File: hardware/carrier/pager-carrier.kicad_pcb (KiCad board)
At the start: 2 copper layers, 97 parts, among them J10 HAPTIC, J11 EXT_LED, J12 PIEZ, J13 USB4235, J14 BATTERY, J5 PANEL, J9 CARDKB, M2 Walter, Q2 AO3401A, Q6 UMH3N, Q7 AO3400A, Q8 MMBT3904, SW3 SKQGAFE010, SW4 JS102011SAQN, U12 CP2102N-A02-GQFN24, U13 SN74LVC2G126DCUR, U14 DRV2605LDGSR, U15 LIS2DW12TR, U16 MAX17048G+T10, U2 BQ25185DLHR, U4 TPS62840DLCR

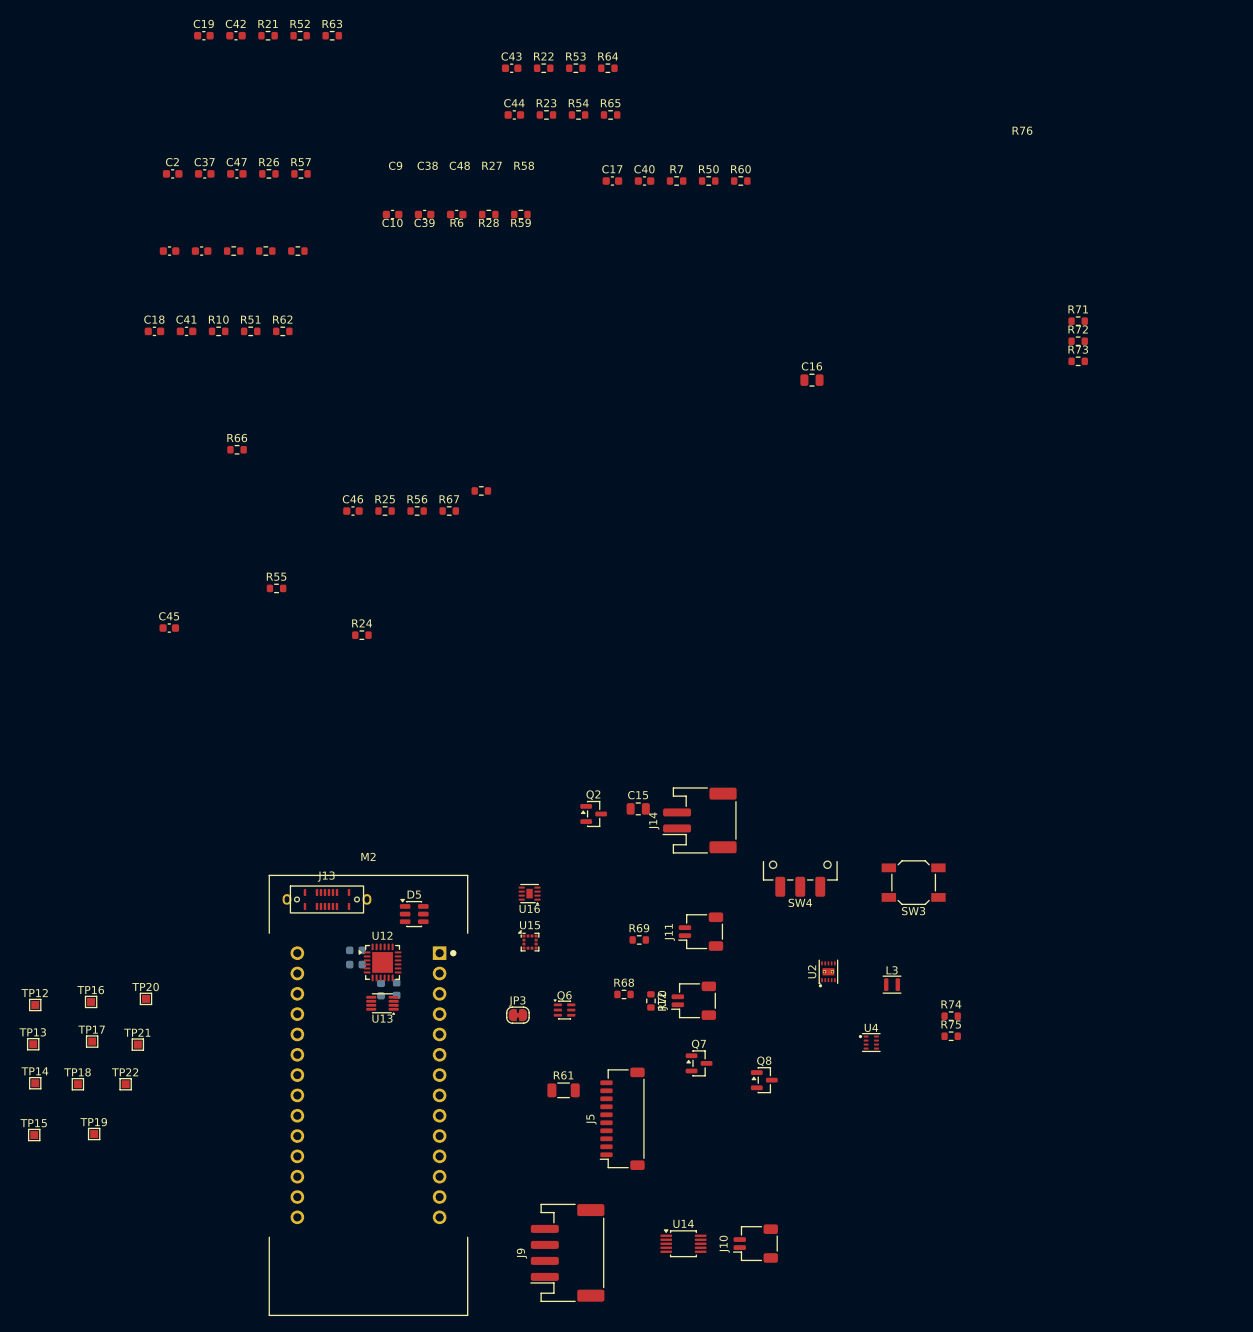
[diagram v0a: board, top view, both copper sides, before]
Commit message: Attempt to layout the PCB
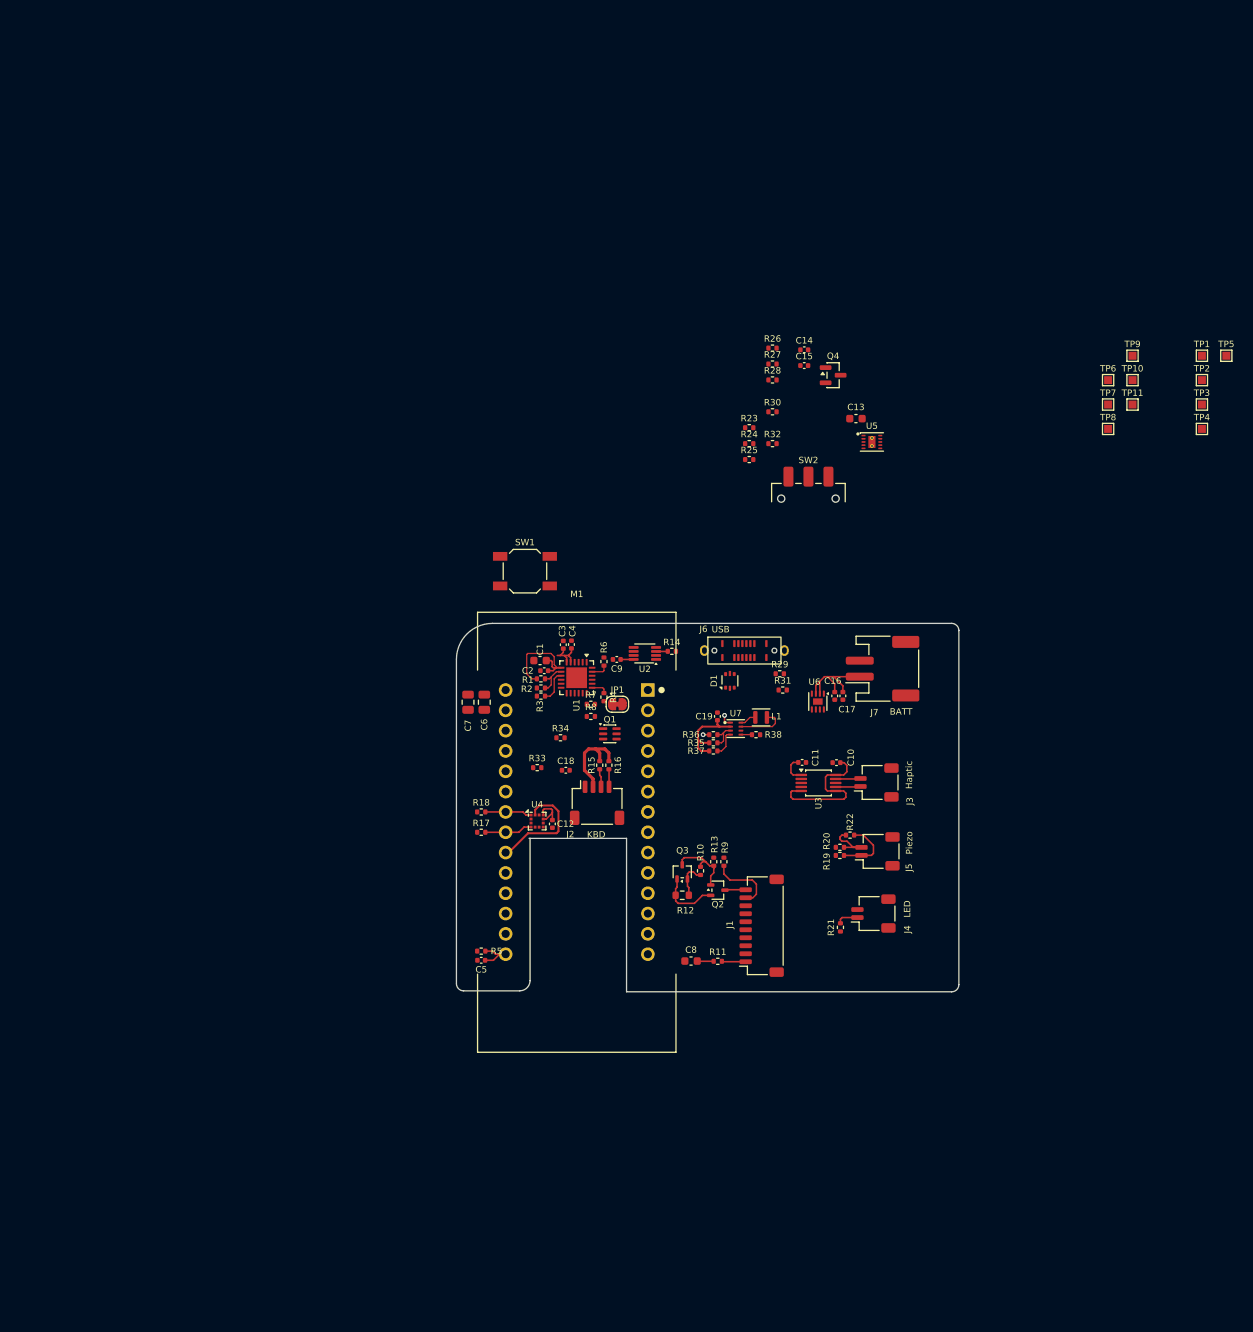
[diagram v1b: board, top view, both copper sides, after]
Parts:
- removed C33, C36: 4.7uF, Capacitor_SMD:C_0603_1608Metric
- removed C34, C35, C37, C39, C42, C45, C46: 100nF, Capacitor_SMD:C_0603_1608Metric
- removed C38, C40, C43, C47, C48: 10uF, Capacitor_SMD:C_0603_1608Metric
- removed C41, C44: 1uF, Capacitor_SMD:C_0603_1608Metric
- removed D5: USBLC6-2SC6, Package_TO_SOT_SMD:SOT-23-6
- removed J10: HAPTIC, Connector_JST:JST_SH_SM02B-SRSS-TB_1x02-1MP_P1.00mm_Horizontal
- removed J11: EXT_LED, Connector_JST:JST_SH_SM02B-SRSS-TB_1x02-1MP_P1.00mm_Horizontal
- removed J12: PIEZ, Connector_JST:JST_SH_SM02B-SRSS-TB_1x02-1MP_P1.00mm_Horizontal
- removed J13: USB4235, pager-carrier:USB_C_Receptacle_GCT_USB4235_Vertical
- removed J14: BATTERY, Connector_JST:JST_PH_S2B-PH-SM4-TB_1x02-1MP_P2.00mm_Horizontal
- removed J9: CARDKB, Connector_JST:JST_PH_S4B-PH-SM4-TB_1x04-1MP_P2.00mm_Horizontal
- removed JP3: auto-boot, Jumper:SolderJumper-2_P1.3mm_Bridged_RoundedPad1.0x1.5mm
- removed L3: 2.2uH, Inductor_SMD:L_Murata_DFE201610P
- removed M2: Walter, pager-carrier:Walter_Module_2x14_THT
- removed Q6: UMH3N, Package_TO_SOT_SMD:SOT-363_SC-70-6
- removed Q7: AO3400A, Package_TO_SOT_SMD:SOT-23
- removed Q8: MMBT3904, Package_TO_SOT_SMD:SOT-23
- removed R50: 22.1k, Resistor_SMD:R_0603_1608Metric
- removed R51: 47.5k, Resistor_SMD:R_0603_1608Metric
- removed R52, R58: 1k, Resistor_SMD:R_0603_1608Metric
- removed R53, R54, R55, R59, R72, R75: 100k, Resistor_SMD:R_0603_1608Metric
- removed R56, R57, R62: 10k, Resistor_SMD:R_0603_1608Metric
- removed R60: 15R, Resistor_SMD:R_0603_1608Metric
- removed R61: 0R, Resistor_SMD:R_1206_3216Metric
- removed R63, R64, R65, R66: 4.7k, Resistor_SMD:R_0603_1608Metric
- removed R67, R68: 220R, Resistor_SMD:R_0603_1608Metric
- removed R69: 330R, Resistor_SMD:R_0603_1608Metric
- removed R70: 1M, Resistor_SMD:R_0603_1608Metric
- removed R71: 56k, Resistor_SMD:R_0603_1608Metric
- removed R73, R74: 0R, Resistor_SMD:R_0603_1608Metric
- removed R76: 267k, Resistor_SMD:R_0603_1608Metric
- removed SW3: SKQGAFE010, Button_Switch_SMD:SW_SPST_SKQG_WithoutStem
- removed SW4: JS102011SAQN, Button_Switch_SMD:SW_SPDT_CK_JS102011SAQN
- removed TP12: AWK_EN_N, TestPoint:TestPoint_Pad_1.0x1.0mm
- removed TP13: TP_IO1, TestPoint:TestPoint_Pad_1.0x1.0mm
- removed TP14: TP_IO5, TestPoint:TestPoint_Pad_1.0x1.0mm
- removed TP15: FL_BTN, TestPoint:TestPoint_Pad_1.0x1.0mm
- removed TP16: 3V3_AWK, TestPoint:TestPoint_Pad_1.0x1.0mm
- removed TP17: GND, TestPoint:TestPoint_Pad_1.0x1.0mm
- removed TP18: VBUS, TestPoint:TestPoint_Pad_1.0x1.0mm
- removed TP19: SYS, TestPoint:TestPoint_Pad_1.0x1.0mm
- removed TP20: SYS_SW, TestPoint:TestPoint_Pad_1.0x1.0mm
- removed TP21: VBAT, TestPoint:TestPoint_Pad_1.0x1.0mm
- removed TP22: 3V3, TestPoint:TestPoint_Pad_1.0x1.0mm
- removed U12: CP2102N-A02-GQFN24, Package_DFN_QFN:QFN-24-1EP_4x4mm_P0.5mm_EP2.6x2.6mm
- removed U13: SN74LVC2G126DCUR, Package_SO:VSSOP-8_2.3x2mm_P0.5mm
- removed U14: DRV2605LDGSR, Package_SO:TSSOP-10_3x3mm_P0.5mm
- removed U15: LIS2DW12TR, Package_LGA:LGA-12_2x2mm_P0.5mm
- removed U16: MAX17048G+T10, Package_DFN_QFN:TDFN-8-1EP_2x2mm_P0.5mm_EP0.8x1.2mm
- added C1: 4.7uF, Capacitor_SMD:C_0603_1608Metric, F.Cu at (82.2, 63.2)
- added C11: 1uF, Capacitor_SMD:C_0402_1005Metric, F.Cu at (114.9, 76.0)
- added C12: 100nF, Capacitor_SMD:C_0402_1005Metric, F.Cu at (83.7, 83.7)
- added C13: 1uF/25V, Capacitor_SMD:C_0603_1608Metric, F.Cu at (121.6, 33.0)
- added C14: 22nF, Capacitor_SMD:C_0402_1005Metric, F.Cu at (115.2, 24.4)
- added C3: 100nF, Capacitor_SMD:C_0402_1005Metric, F.Cu at (85.1, 61.3)
- added C4: 4.7uF, Capacitor_SMD:C_0402_1005Metric, F.Cu at (86.1, 61.2)
- added C5: 100nF, Capacitor_SMD:C_0402_1005Metric, F.Cu at (74.8, 100.7)
- added C6: 100uF, Capacitor_SMD:C_0805_2012Metric, F.Cu at (75.2, 68.5)
- added C7: 100uF, Capacitor_SMD:C_0805_2012Metric, F.Cu at (73.2, 68.5)
- added C8: 10uF, Capacitor_SMD:C_0603_1608Metric, F.Cu at (101.0, 100.8)
- added D1: USBLC6-2P6, Package_TO_SOT_SMD:SOT-666, F.Cu at (105.9, 65.8)
- added J1: PANEL, Connector_JST:JST_SH_SM10B-SRSS-TB_1x10-1MP_P1.00mm_Horizontal, F.Cu at (109.9, 96.4)
- added J2: CARDKB, Connector_JST:JST_SH_SM04B-SRSS-TB_1x04-1MP_P1.00mm_Horizontal, F.Cu at (89.3, 81.0)
- added J3: HAPTIC, Connector_JST:JST_SH_SM02B-SRSS-TB_1x02-1MP_P1.00mm_Horizontal, F.Cu at (124.2, 78.5)
- added J4: EXT_LED, Connector_JST:JST_SH_SM02B-SRSS-TB_1x02-1MP_P1.00mm_Horizontal, F.Cu at (123.8, 94.9)
- added J6: USB4235, pager-carrier:USB_C_Receptacle_GCT_USB4235_Vertical, F.Cu at (107.7, 62.0)
- added J7: BATTERY, Connector_JST:JST_PH_S2B-PH-SM4-TB_1x02-1MP_P2.00mm_Horizontal, F.Cu at (125.0, 64.3)
- added JP1: auto-boot, Jumper:SolderJumper-2_P1.3mm_Bridged_RoundedPad1.0x1.5mm, F.Cu at (91.8, 68.7)
- added L1: 2.2uH, Inductor_SMD:L_Murata_DFE201610P, F.Cu at (109.8, 70.4)
- added M1: Walter, pager-carrier:Walter_Module_2x14_THT, F.Cu at (86.7, 83.4)
- added Q1: UMH3N, Package_TO_SOT_SMD:SOT-363_SC-70-6, F.Cu at (90.9, 72.4)
- added Q3: MMST3904, Package_TO_SOT_SMD:SOT-323_SC-70, F.Cu at (99.9, 89.7)
- added Q4: AO3401A, Package_TO_SOT_SMD:SOT-23, F.Cu at (118.8, 27.6)
- added R1: 22.1k, Resistor_SMD:R_0402_1005Metric, F.Cu at (82.3, 65.5)
- added R11: 0R, Resistor_SMD:R_0402_1005Metric, F.Cu at (104.4, 100.8)
- added R12: 15R, Resistor_SMD:R_0603_1608Metric, F.Cu at (99.9, 92.6)
- added R13: 0R, Resistor_SMD:R_0402_1005Metric, F.Cu at (105.1, 88.4)
- added R14: 10k, Resistor_SMD:R_0402_1005Metric, F.Cu at (98.6, 62.1)
- added R15: 4.7k, Resistor_SMD:R_0402_1005Metric, F.Cu at (89.6, 76.3)
- added R16: 4.7k, Resistor_SMD:R_0402_1005Metric, F.Cu at (90.8, 76.3)
- added R17: 4.7k, Resistor_SMD:R_0402_1005Metric, F.Cu at (74.8, 84.7)
- added R18: 4.7k, Resistor_SMD:R_0402_1005Metric, F.Cu at (74.8, 82.2)
- added R19: 220R, Resistor_SMD:R_0402_1005Metric, F.Cu at (119.6, 87.6)
- added R2: 47.5k, Resistor_SMD:R_0402_1005Metric, F.Cu at (82.3, 66.7)
- added R20: 220R, Resistor_SMD:R_0402_1005Metric, F.Cu at (119.6, 86.6)
- added R29: 5.1k, Resistor_SMD:R_0402_1005Metric, F.Cu at (112.1, 64.9)
- added R3: 1k, Resistor_SMD:R_0402_1005Metric, F.Cu at (82.3, 67.7)
- added R30: 10k, Resistor_SMD:R_0402_1005Metric, F.Cu at (111.2, 32.2)
- added R31: 5.1k, Resistor_SMD:R_0402_1005Metric, F.Cu at (112.5, 66.9)
- added R32: 2.2M, Resistor_SMD:R_0402_1005Metric, F.Cu at (111.2, 36.1)
- added R33: 56k, Resistor_SMD:R_0402_1005Metric, F.Cu at (81.8, 76.6)
- added R34: 100k, Resistor_SMD:R_0402_1005Metric, F.Cu at (84.7, 72.9)
- added R35: 0R, Resistor_SMD:R_0402_1005Metric, F.Cu at (103.8, 73.5)
- added R36: 0R, Resistor_SMD:R_0402_1005Metric, F.Cu at (103.8, 72.5)
- added R37: 100k, Resistor_SMD:R_0402_1005Metric, F.Cu at (103.8, 74.5)
- added R38: 267k, Resistor_SMD:R_0402_1005Metric, F.Cu at (109.2, 72.5)
- added R4: 100k, Resistor_SMD:R_0402_1005Metric, F.Cu at (90.1, 67.8)
- added R5: 100k, Resistor_SMD:R_0402_1005Metric, F.Cu at (74.8, 99.6)
- added R8: 10k, Resistor_SMD:R_0402_1005Metric, F.Cu at (88.5, 70.2)
- added R9: 1k, Resistor_SMD:R_0402_1005Metric, F.Cu at (103.9, 88.4)
- added SW1: SKQGAFE010, Button_Switch_SMD:SW_SPST_SKQG_WithoutStem, F.Cu at (80.3, 52.1)
- added SW2: JS102011SAQN, Button_Switch_SMD:SW_SPDT_CK_JS102011SAQN, F.Cu at (115.7, 43.0)
- added TP1: AWK_EN_N, TestPoint:TestPoint_Pad_1.0x1.0mm, F.Cu at (164.9, 25.1)
- added TP10: VBAT, TestPoint:TestPoint_Pad_1.0x1.0mm, F.Cu at (156.2, 28.2)
- added TP11: 3V3, TestPoint:TestPoint_Pad_1.0x1.0mm, F.Cu at (156.2, 31.2)
- added TP2: TP_IO1, TestPoint:TestPoint_Pad_1.0x1.0mm, F.Cu at (164.9, 28.2)
- added TP3: TP_IO5, TestPoint:TestPoint_Pad_1.0x1.0mm, F.Cu at (164.9, 31.2)
- added TP4: FL_BTN, TestPoint:TestPoint_Pad_1.0x1.0mm, F.Cu at (164.9, 34.3)
- added TP5: 3V3_AWK, TestPoint:TestPoint_Pad_1.0x1.0mm, F.Cu at (167.9, 25.1)
- added TP6: GND, TestPoint:TestPoint_Pad_1.0x1.0mm, F.Cu at (153.2, 28.2)
- added TP7: VBUS, TestPoint:TestPoint_Pad_1.0x1.0mm, F.Cu at (153.2, 31.2)
- added TP8: SYS, TestPoint:TestPoint_Pad_1.0x1.0mm, F.Cu at (153.2, 34.3)
- added TP9: SYS_SW, TestPoint:TestPoint_Pad_1.0x1.0mm, F.Cu at (156.2, 25.1)
- added U1: CP2102N-A02-GQFN24, Package_DFN_QFN:QFN-24-1EP_4x4mm_P0.5mm_EP2.6x2.6mm, F.Cu at (86.7, 65.4)
- added U3: DRV2605LDGSR, Package_SO:TSSOP-10_3x3mm_P0.5mm, F.Cu at (117.0, 78.5)
- added U5: BQ25185DLHR, pager-carrier:BQ25185_WSON-10_DLH0010A_2.2x2mm_P0.4mm_EP0.9x1.5mm, F.Cu at (123.6, 35.9)
- added U6: MAX17048G+T10, Package_DFN_QFN:TDFN-8-1EP_2x2mm_P0.5mm_EP0.8x1.2mm, F.Cu at (116.9, 68.4)
- added U7: TPS62840DLCR, pager-carrier:TPS62840_VSON-HR-8_DLC0008B_1.5x2mm_P0.5mm, F.Cu at (106.6, 71.8)
- C10: value 22nF -> 1uF; footprint Capacitor_SMD:C_0603_1608Metric -> Capacitor_SMD:C_0402_1005Metric
- C15, C16: value 100uF -> 10uF; footprint Capacitor_SMD:C_0805_2012Metric -> Capacitor_SMD:C_0402_1005Metric
- C17, C18: value 10uF -> 100nF; footprint Capacitor_SMD:C_0603_1608Metric -> Capacitor_SMD:C_0402_1005Metric
- C19, C2: footprint Capacitor_SMD:C_0603_1608Metric -> Capacitor_SMD:C_0402_1005Metric
- C9: value 1uF/25V -> 100nF; footprint Capacitor_SMD:C_0603_1608Metric -> Capacitor_SMD:C_0402_1005Metric
- J5: value PANEL -> PIEZ; footprint Connector_JST:JST_SH_SM10B-SRSS-TB_1x10-1MP_P1.00mm_Horizontal -> Connector_JST:JST_SH_SM02B-SRSS-TB_1x02-1MP_P1.00mm_Horizontal
- Q2: value AO3401A -> SI1308EDL; footprint Package_TO_SOT_SMD:SOT-23 -> Package_TO_SOT_SMD:SOT-323_SC-70
- R10: value 10k -> 100k; footprint Resistor_SMD:R_0603_1608Metric -> Resistor_SMD:R_0402_1005Metric
- R21: value 0R -> 330R; footprint Resistor_SMD:R_0603_1608Metric -> Resistor_SMD:R_0402_1005Metric
- R22: value 18k -> 1M; footprint Resistor_SMD:R_0603_1608Metric -> Resistor_SMD:R_0402_1005Metric
- R23: value 10k -> 0R; footprint Resistor_SMD:R_0603_1608Metric -> Resistor_SMD:R_0402_1005Metric
- R24: value 604R -> 10k; footprint Resistor_SMD:R_0603_1608Metric -> Resistor_SMD:R_0402_1005Metric
- R25: value 10k -> 18k; footprint Resistor_SMD:R_0603_1608Metric -> Resistor_SMD:R_0402_1005Metric
- R26: footprint Resistor_SMD:R_0603_1608Metric -> Resistor_SMD:R_0402_1005Metric
- R27: value 5.1k -> 604R; footprint Resistor_SMD:R_0603_1608Metric -> Resistor_SMD:R_0402_1005Metric
- R28: value 2.2M -> 10k; footprint Resistor_SMD:R_0603_1608Metric -> Resistor_SMD:R_0402_1005Metric
- R6: value 0R -> 100k; footprint Resistor_SMD:R_0603_1608Metric -> Resistor_SMD:R_0402_1005Metric
- R7: value 5.1k -> 10k; footprint Resistor_SMD:R_0603_1608Metric -> Resistor_SMD:R_0402_1005Metric
- U2: value BQ25185DLHR -> SN74LVC2G126DCUR; footprint pager-carrier:BQ25185_WSON-10_DLH0010A_2.2x2mm_P0.4mm_EP0.9x1.5mm -> Package_SO:VSSOP-8_2.3x2mm_P0.5mm
- U4: value TPS62840DLCR -> LIS2DW12TR; footprint pager-carrier:TPS62840_VSON-HR-8_DLC0008B_1.5x2mm_P0.5mm -> Package_LGA:LGA-12_2x2mm_P0.5mm
- moved R21 132.4 mm to (119.7, 96.6), turned to 90 degrees
- moved C19 106.6 mm to (104.3, 70.2), turned to 90 degrees
- moved C10 105.1 mm to (119.2, 76.0), turned to 180 degrees
- moved R22 103.2 mm to (120.9, 85.1)
- moved R10 90.4 mm to (102.2, 89.5), turned to -90 degrees
- moved C2 77.6 mm to (82.7, 64.5), turned to 180 degrees
- moved C18 75.2 mm to (85.4, 77.0)
- moved C17 70.5 mm to (120.0, 67.7), turned to -90 degrees
- moved R6 69.1 mm to (90.1, 63.4), turned to 90 degrees
- moved R26 66.6 mm to (111.2, 24.2)
- moved R7 66.3 mm to (88.5, 68.7)
- moved R28 65.4 mm to (111.2, 28.2)
- moved C9 62.3 mm to (91.7, 63.1), turned to 180 degrees
- moved C15 59.2 mm to (115.2, 26.4)
- moved R24 54.0 mm to (108.3, 36.1)
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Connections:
- C10 pad 1: Net-(Q2-G) -> 3V3_AWK
- C10 pad 2: SYS -> GND
- C15 pad 1: SYS_SW -> SYS
- C16 pad 1: SYS_SW -> VBAT
- C17 pad 1: SYS_SW -> VBAT
- C18 pad 1: SYS -> VBUS_DET
- C19 pad 1: VBAT -> SYS_SW
- C2 pad 1: VBUS_DET -> VBUS
- C9 pad 1: Net-(U2-IN) -> /Core/BRG_3V3
- J5 pad 2: GND -> Net-(J5-Pin_2)
- Q2 pad 2: SYS -> Net-(Q2-S)
- Q2 pad 3: SYS_SW -> /Core/FL_N
- R10 pad 1: Net-(U2-TS/MR) -> Net-(Q2-G)
- R21 pad 1: 3V3 -> /Core/EXT_LED
- R21 pad 2: Net-(J5-Pin_1) -> Net-(J4-Pin_1)
- R22 pad 1: Net-(U2-ILIM/VSET) -> Net-(J5-Pin_2)
- R22 pad 2: GND -> Net-(J5-Pin_1)
- R23 pad 1: 3V3 -> VBUS
- R23 pad 2: CHG_STAT1 -> Net-(U5-IN)
- R24 pad 1: Net-(U2-ISET) -> Net-(U5-TS/MR)
- R25 pad 1: 3V3 -> Net-(U5-ILIM/VSET)
- R25 pad 2: CHG_STAT2 -> GND
- R26 pad 1: Net-(SW4-B) -> 3V3
- R26 pad 2: Net-(Q2-G) -> CHG_STAT1
- R28 pad 1: Net-(Q2-G) -> 3V3
- R28 pad 2: SYS -> CHG_STAT2
- R6 pad 1: VBUS -> Net-(Q1B-E2)
- R6 pad 2: Net-(U2-IN) -> GND
- R7 pad 1: Net-(J13-CC2) -> Net-(Q1B-E2)
- R7 pad 2: GND -> Net-(Q1A-B1)
- U2 pad 1: SYS -> VBUS_DET
- U2 pad 2: VBAT -> /Core/ESP_TX0
- U2 pad 3: CHG_STAT2 -> /Core/ESP_RX0
- U2 pad 5: GND -> /Core/BRG_TXD
- U2 pad 6: Net-(U2-TS/MR) -> /Core/BRG_RXD
- U2 pad 7: Net-(U2-ILIM/VSET) -> VBUS_DET
- U2 pad 8: Net-(U2-ISET) -> /Core/BRG_3V3
- U4 pad 1: GND -> AON_SCL
- U4 pad 2: SYS_SW -> 3V3
- U4 pad 3: Net-(U4-MODE) -> GND
- U4 pad 4: Net-(U4-EN) -> AON_SDA
- U4 pad 5: Net-(U4-VSET) -> unconnected-(U4-NC-Pad5)
- U4 pad 7: Net-(U4-SW) -> GND
- U4 pad 8: 3V3 -> GND
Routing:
- net 3V3_AWK: track 0.00 -> 29.4 mm
- net /Core/ACC_INT1: track 0.00 -> 14.3 mm
- net VBAT: track 0.00 -> 13.3 mm
- net VBUS: track 0.00 -> 13.0 mm
- net SYS_SW: track 0.00 -> 10.4 mm
- net Net-(Q2-G): track 0.00 -> 9.15 mm
- net 3V3: track 0.00 -> 8.89 mm
- net /Core/FL_P: track 0.00 -> 8.48 mm
- net Net-(J5-Pin_1): track 0.00 -> 7.74 mm
- net Net-(Q2-S): track 0.00 -> 7.74 mm
- net GND: track 0.00 -> 6.99 mm, vias 0 -> 2
- net /Core/BRG_3V3: track 0.32 -> 7.01 mm
- net Net-(J5-Pin_2): track 0.00 -> 6.42 mm
- net Net-(U7-SW): track 0.00 -> 6.20 mm
- net AON_SDA: track 0.00 -> 5.98 mm
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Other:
- board outline added: 62.8 x 46 mm
- board text added: "BATT"
- board text added: "Haptic"
- board text added: "KBD"
- board text added: "LED"
- board text added: "Piezo"
- board text added: "USB"
